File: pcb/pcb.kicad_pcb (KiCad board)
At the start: 2 copper layers, 75 x 75 mm, 36 parts, among them J1 Connector, USB-TYPE-C-16P, SW1 SW_Push, U4 NCP1117-3.3_SOT223, X1 X322512MSB4SI

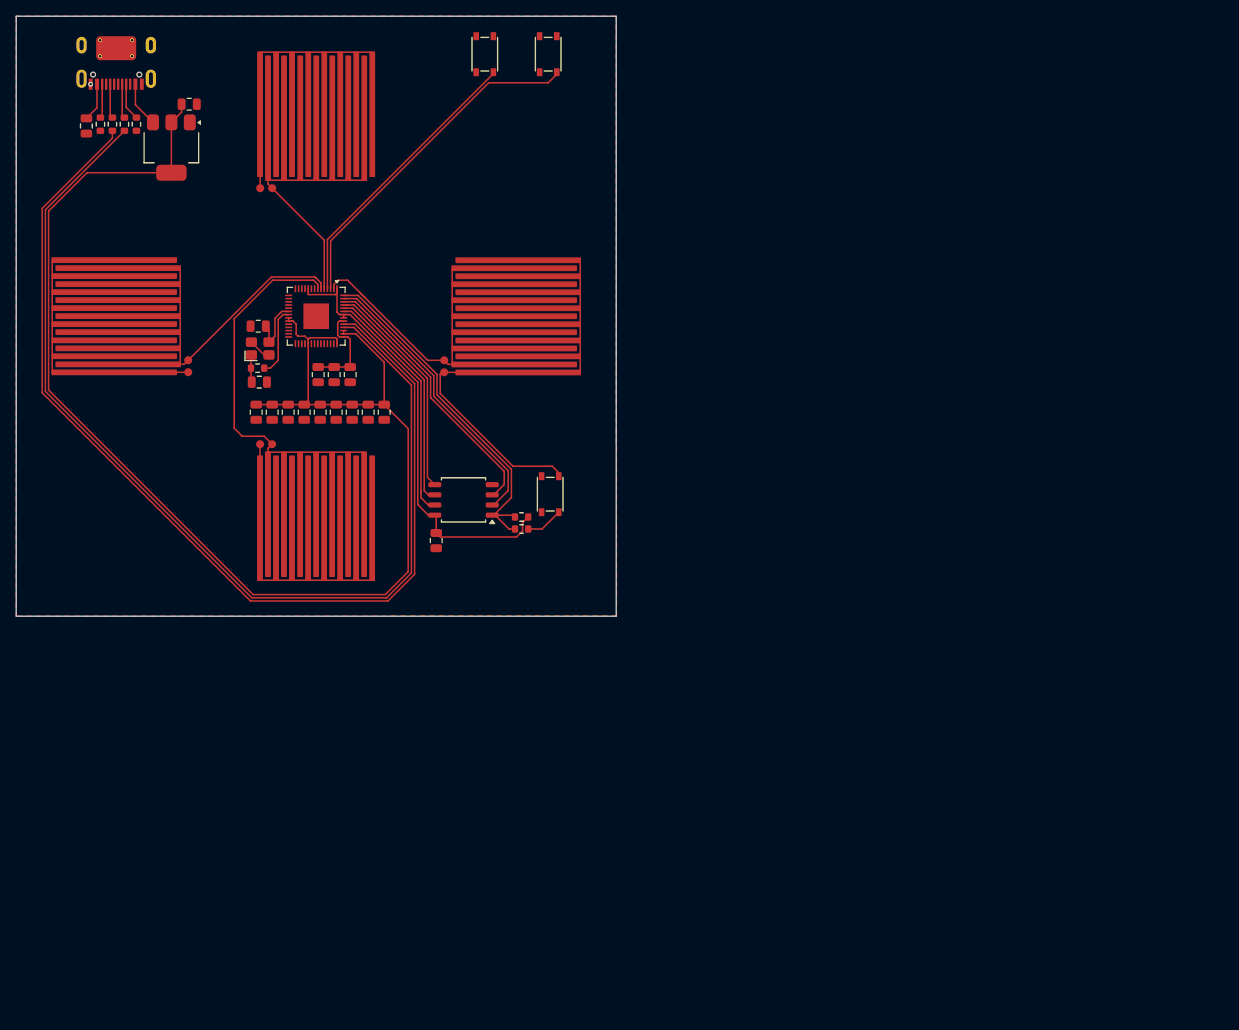
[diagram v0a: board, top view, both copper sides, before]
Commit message: still working on it LOL
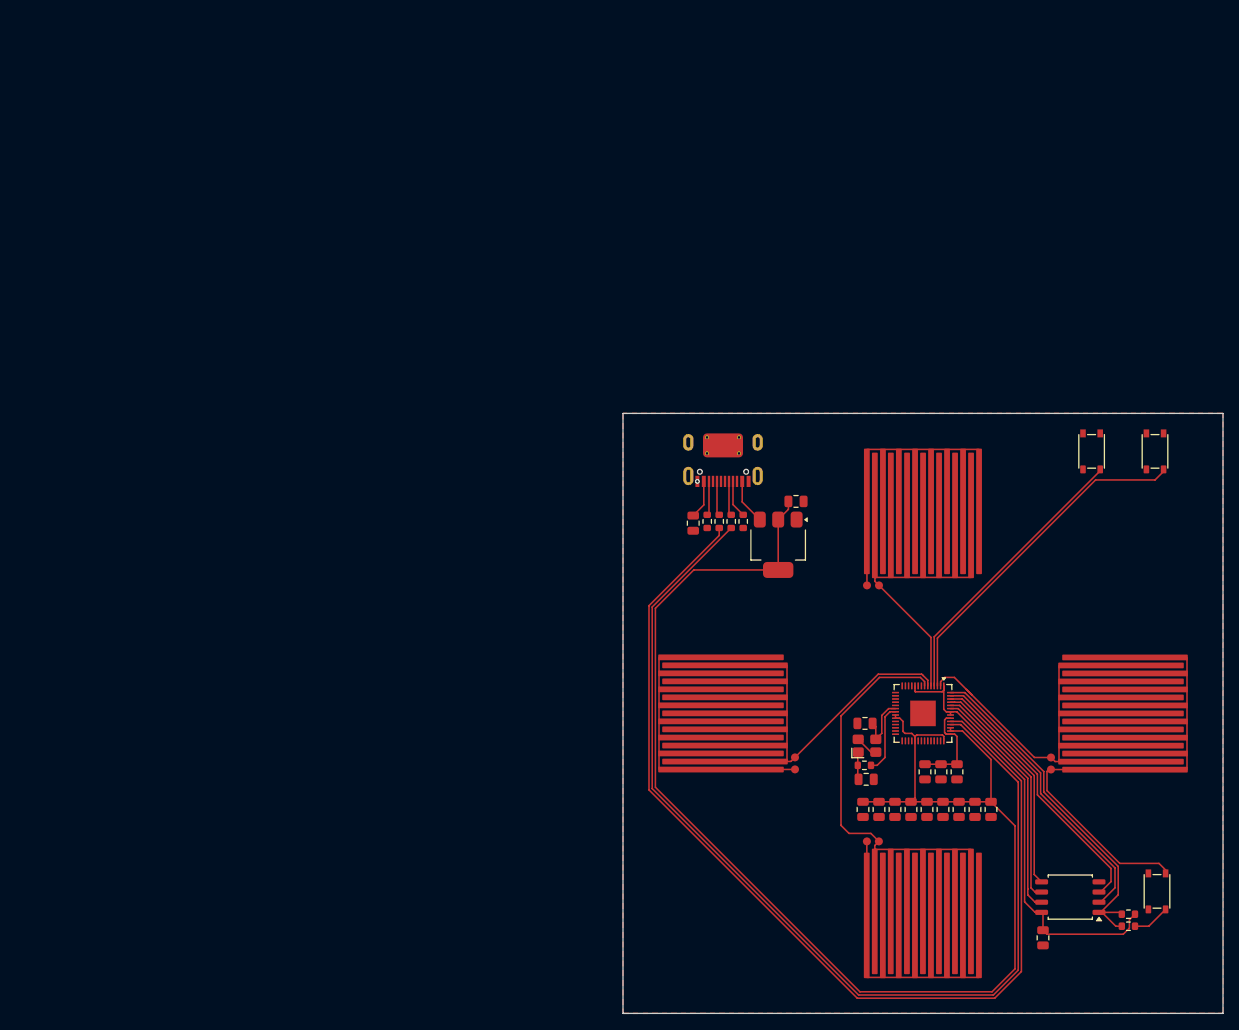
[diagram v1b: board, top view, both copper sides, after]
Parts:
- moved C17 90.7 mm to (106.2, 95.4)
- moved R5 90.7 mm to (139.0, 112.2)
- moved R6 90.7 mm to (139.0, 113.8)
- moved R7 90.7 mm to (106.0, 93.6)
- moved SW_Menu1 90.7 mm to (134.4, 54.4)
- moved C1 90.7 mm to (84.6, 63.4)
- moved C10 90.7 mm to (117.8, 99.2)
- moved C11 90.7 mm to (119.8, 99.2)
- moved C12 90.7 mm to (121.8, 99.2)
- moved C13 90.7 mm to (113.6, 94.5)
- moved C14 90.7 mm to (115.6, 94.5)
- moved C15 90.7 mm to (117.6, 94.5)
- moved C16 90.7 mm to (106.1, 88.4)
- moved C2 90.7 mm to (97.5, 60.6)
- moved C3 90.7 mm to (128.3, 115.2)
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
